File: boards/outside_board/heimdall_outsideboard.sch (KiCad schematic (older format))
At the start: 11 parts, among them J1 Conn_01x09, J2 Conn_01x06, Q1 2N3904, Q2 2N7000

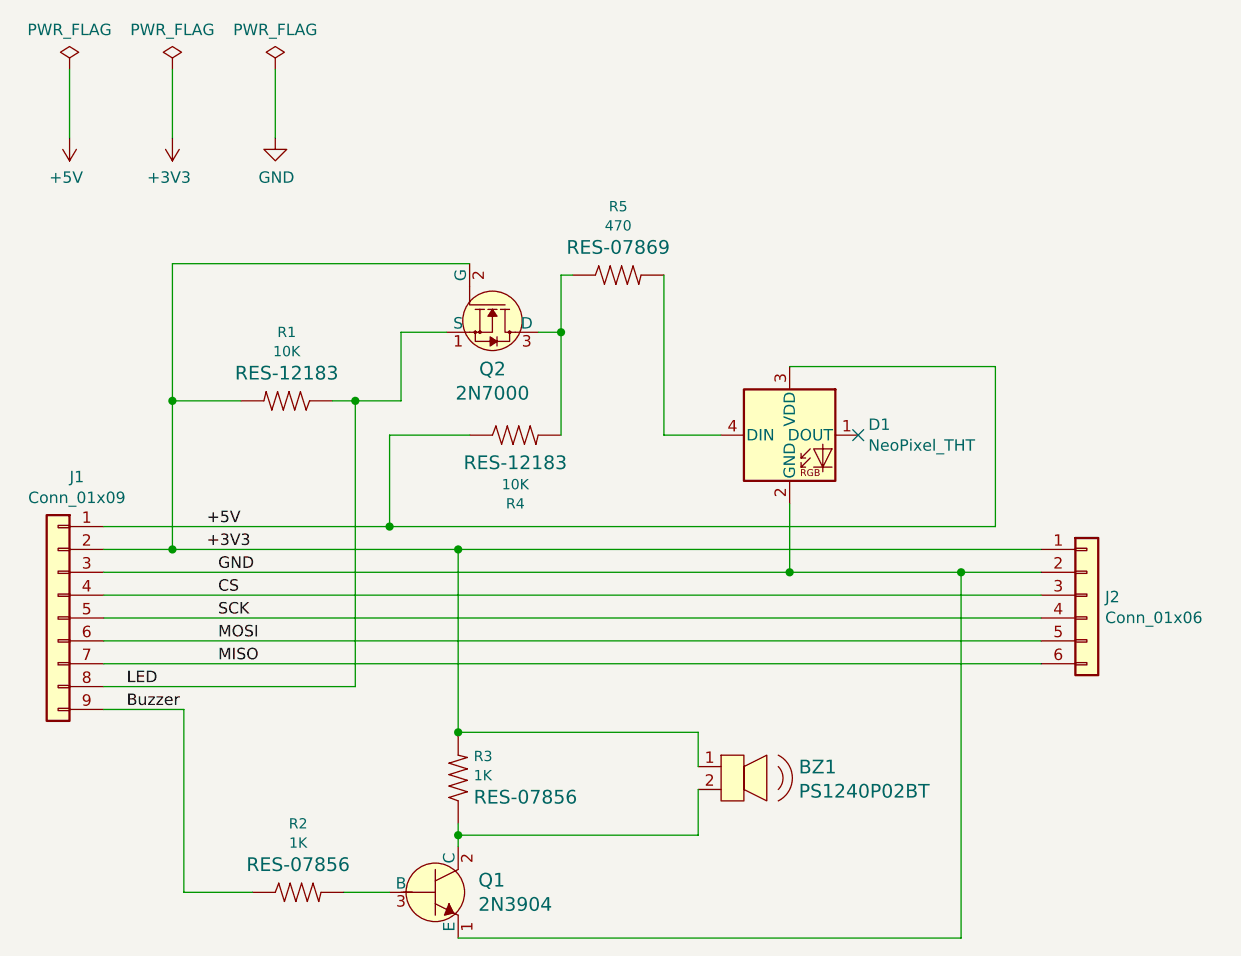
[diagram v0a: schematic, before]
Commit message: Update outside board schematics and layout to revision 2
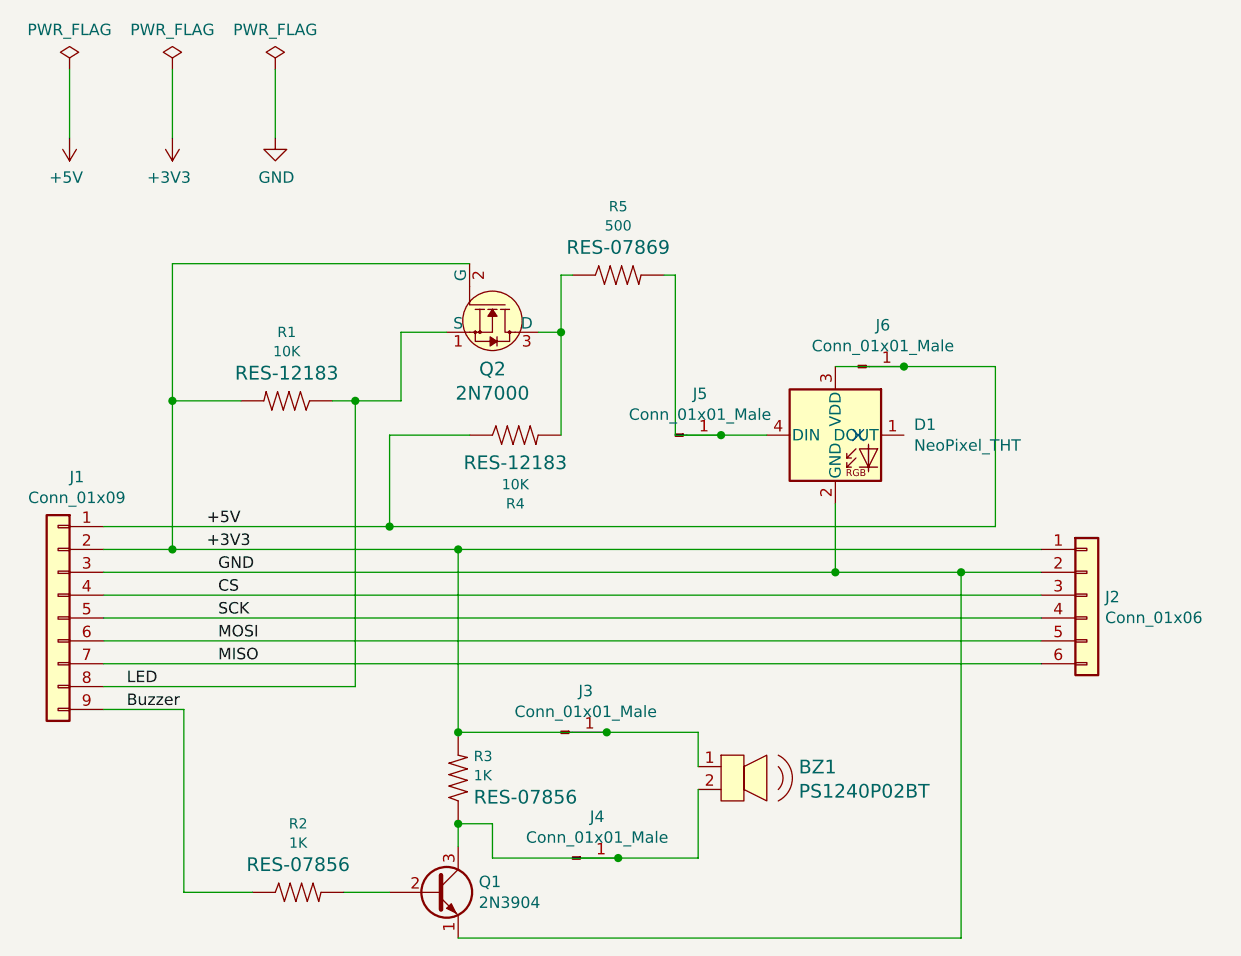
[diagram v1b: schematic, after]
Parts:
- removed Q1: 2N3904, Package_TO_SOT_THT:TO-92_Inline, symbol dk_Transistors-Bipolar-BJT-Single:2N3904
- added J3, J4, J5, J6: Conn_01x01_Male, Connector_PinHeader_2.54mm:PinHeader_1x01_P2.54mm_Vertical, symbol Connector:Conn_01x01_Male
- added Q1: 2N3904, Package_TO_SOT_THT:TO-92_Inline, symbol Transistor_BJT:2N3904
- D1: footprint LED:WS2812B -> LED_THT:LED_D5.0mm-4_RGB
- R5: value 470 -> 500
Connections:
- net +3V3: now also J3.1 (Pin_1)
- net +5V: now also J6.1 (Pin_1)
- net GND: now also Q1.1 (E)
- net at D1.4 (DIN), R5.2: now also J5.1 (Pin_1)
- net at BZ1.2, R3.1: now also J4.1 (Pin_1), Q1.3 (C)
- net at R2.2: now also Q1.2 (B)
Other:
- moved on the sheet: D1
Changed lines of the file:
@@
 Sheet 1 1
 Title "Heimdall Outside Board"
-Date "2020-07-24"
-Rev "01"
+Date "2020-11-07"
+Rev "02"
 Comp ""
 Comment1 "https://opensource.org/licenses/MIT"
@@
 L LED:NeoPixel_THT D1
 U 1 1 5F17E8A3
-P 4350 4950
-F 0 "D1" H 4694 4996 50  0000 L CNN
-F 1 "NeoPixel_THT" H 4694 4905 50  0000 L CNN
-F 2 "LED:WS2812B" H 4400 4650 50  0001 L TNN
-F 3 "https://www.adafruit.com/product/1938" H 4450 4575 50  0001 L TNN
-	1    4350 4950
+P 4550 4950
+F 0 "D1" H 4894 4996 50  0000 L CNN
+F 1 "NeoPixel_THT" H 4894 4905 50  0000 L CNN
+F 2 "LED_THT:LED_D5.0mm-4_RGB" H 4600 4650 50  0001 L TNN
+F 3 "https://www.adafruit.com/product/1938" H 4650 4575 50  0001 L TNN
+	1    4550 4950
 	1    0    0    -1
 $EndComp
@@
 	1700 6950 2000 6950
 Wire Wire Line
-	2900 6750 2900 6700
-Wire Wire Line
 	2900 6250 2900 5450
-Wire Wire Line
-	2900 6250 3950 6250
-Wire Wire Line
-	3950 6250 3950 6400
-Connection ~ 2900 6250
-Wire Wire Line
-	3950 6500 3950 6700
-Wire Wire Line
-	3950 6700 2900 6700
-Connection ~ 2900 6700
-Wire Wire Line
-	2900 6700 2900 6650
 Wire Wire Line
 	5100 7150 5100 5550
@@
 Connection ~ 3350 4500
 Wire Wire Line
-	3800 4250 3800 4950
-Wire Wire Line
-	3800 4950 4050 4950
-Wire Wire Line
 	2850 4500 2650 4500
-$Comp
-L SparkFun-Resistors:470OHM-0603-1_10W-1% R5
-U 1 1 5F209E6B
-P 3600 4250
-F 0 "R5" H 3600 4550 45  0000 C CNN
-F 1 "470" H 3600 4466 45  0000 C CNN
-F 2 "Resistor_THT:R_Axial_DIN0207_L6.3mm_D2.5mm_P10.16mm_Horizontal" H 3600 4400 20  0001 C CNN
-F 3 "" H 3600 4250 60  0001 C CNN
-F 4 "RES-07869" H 3600 4371 60  0000 C CNN "Field4"
-	1    3600 4250
-	1    0    0    -1
-$EndComp
 Wire Wire Line
 	1350 5450 1650 5450
@@
 Wire Wire Line
 	5250 5350 5250 4650
-Wire Wire Line
-	5250 4650 4350 4650
-Wire Wire Line
-	1350 5550 4350 5550
-Wire Wire Line
-	4350 5550 4350 5250
-Connection ~ 4350 5550
-Wire Wire Line
-	4350 5550 5100 5550
 $Comp
 L power:PWR_FLAG #FLG01
@@
 F 3 "~" H 2100 3350 50  0001 C CNN
 	1    2100 3350
-	1    0    0    -1
-$EndComp
-$Comp
-L dk_Transistors-Bipolar-BJT-Single:2N3904 Q1
-U 1 1 5F2401CC
-P 2800 6950
-F 0 "Q1" H 2988 7003 60  0000 L CNN
-F 1 "2N3904" H 2988 6897 60  0000 L CNN
-F 2 "Package_TO_SOT_THT:TO-92_Inline" H 3000 7150 60  0001 L CNN
-F 3 "https://my.centralsemi.com/get_document.php?cmp=1&mergetype=pd&mergepath=pd&pdf_id=LSSGP072.PDF" H 3000 7250 60  0001 L CNN
-F 4 "2N3904CS-ND" H 3000 7350 60  0001 L CNN "Digi-Key_PN"
-F 5 "2N3904" H 3000 7450 60  0001 L CNN "MPN"
-F 6 "Discrete Semiconductor Products" H 3000 7550 60  0001 L CNN "Category"
-F 7 "Transistors - Bipolar (BJT) - Single" H 3000 7650 60  0001 L CNN "Family"
-F 8 "https://my.centralsemi.com/get_document.php?cmp=1&mergetype=pd&mergepath=pd&pdf_id=LSSGP072.PDF" H 3000 7750 60  0001 L CNN "DK_Datasheet_Link"
-F 9 "/product-detail/en/central-semiconductor-corp/2N3904/2N3904CS-ND/4806876" H 3000 7850 60  0001 L CNN "DK_Detail_Page"
-F 10 "TRANS NPN 40V TO-92" H 3000 7950 60  0001 L CNN "Description"
-F 11 "Central Semiconductor Corp" H 3000 8050 60  0001 L CNN "Manufacturer"
-F 12 "Active" H 3000 8150 60  0001 L CNN "Status"
-	1    2800 6950
 	1    0    0    -1
 $EndComp
@@
 Wire Wire Line
 	2100 3350 2100 3650
+$Comp
+L Connector:Conn_01x01_Male J3
+U 1 1 5FA614DC
+P 3350 6250
+F 0 "J3" H 3458 6431 50  0000 C CNN
+F 1 "Conn_01x01_Male" H 3458 6340 50  0000 C CNN
+F 2 "Connector_PinHeader_2.54mm:PinHeader_1x01_P2.54mm_Vertical" H 3350 6250 50  0001 C CNN
+F 3 "~" H 3350 6250 50  0001 C CNN
+	1    3350 6250
+	1    0    0    -1
+$EndComp
+$Comp
+L Connector:Conn_01x01_Male J4
+U 1 1 5FA62088
+P 3400 6800
+F 0 "J4" H 3508 6981 50  0000 C CNN
+F 1 "Conn_01x01_Male" H 3508 6890 50  0000 C CNN
+F 2 "Connector_PinHeader_2.54mm:PinHeader_1x01_P2.54mm_Vertical" H 3400 6800 50  0001 C CNN
+F 3 "~" H 3400 6800 50  0001 C CNN
+	1    3400 6800
+	1    0    0    -1
+$EndComp
+$Comp
+L Connector:Conn_01x01_Male J5
+U 1 1 5FA690EE
+P 3850 4950
+F 0 "J5" H 3958 5131 50  0000 C CNN
+F 1 "Conn_01x01_Male" H 3958 5040 50  0000 C CNN
+F 2 "Connector_PinHeader_2.54mm:PinHeader_1x01_P2.54mm_Vertical" H 3850 4950 50  0001 C CNN
+F 3 "~" H 3850 4950 50  0001 C CNN
+	1    3850 4950
+	1    0    0    -1
+$EndComp
+$Comp
+L Connector:Conn_01x01_Male J6
+U 1 1 5FA69F83
+P 4650 4650
+F 0 "J6" H 4758 4831 50  0000 C CNN
+F 1 "Conn_01x01_Male" H 4758 4740 50  0000 C CNN
+F 2 "Connector_PinHeader_2.54mm:PinHeader_1x01_P2.54mm_Vertical" H 4650 4650 50  0001 C CNN
+F 3 "~" H 4650 4650 50  0001 C CNN
+	1    4650 4650
+	1    0    0    -1
+$EndComp
+Wire Wire Line
+	1350 5550 4550 5550
+Wire Wire Line
+	4550 5250 4550 5550
+Connection ~ 4550 5550
+Wire Wire Line
+	4550 5550 5100 5550
+Wire Wire Line
+	3850 4250 3800 4250
+Wire Wire Line
+	4050 4950 4250 4950
+Wire Wire Line
+	4850 4650 5250 4650
+Wire Wire Line
+	2900 6650 2900 6750
+Wire Wire Line
+	3950 6400 3950 6250
+Wire Wire Line
+	3950 6250 3550 6250
+Wire Wire Line
+	3550 6250 2900 6250
+Connection ~ 3550 6250
+Connection ~ 2900 6250
+Wire Wire Line
+	3950 6500 3950 6800
+Wire Wire Line
+	3950 6800 3600 6800
+Wire Wire Line
+	3600 6800 3050 6800
+Wire Wire Line
+	3050 6800 3050 6650
+Wire Wire Line
+	3050 6650 2900 6650
+Connection ~ 3600 6800
+Connection ~ 2900 6650
+Wire Wire Line
+	4850 4650 4550 4650
+Connection ~ 4850 4650
+Wire Wire Line
+	4050 4950 3850 4950
+Wire Wire Line
+	3850 4950 3850 4250
+Connection ~ 4050 4950
+$Comp
+L Transistor_BJT:2N3904 Q1
+U 1 1 5FA8FEA8
+P 2800 6950
+F 0 "Q1" H 2990 6996 50  0000 L CNN
+F 1 "2N3904" H 2990 6905 50  0000 L CNN
+F 2 "Package_TO_SOT_THT:TO-92_Inline" H 3000 6875 50  0001 L CIN
+F 3 "https://www.onsemi.com/pub/Collateral/2N3903-D.PDF" H 2800 6950 50  0001 L CNN
+	1    2800 6950
+	1    0    0    -1
+$EndComp
+$Comp
+L SparkFun-Resistors:470OHM-0603-1_10W-1% R5
+U 1 1 5F209E6B
+P 3600 4250
+F 0 "R5" H 3600 4550 45  0000 C CNN
+F 1 "500" H 3600 4466 45  0000 C CNN
+F 2 "Resistor_THT:R_Axial_DIN0207_L6.3mm_D2.5mm_P10.16mm_Horizontal" H 3600 4400 20  0001 C CNN
+F 3 "" H 3600 4250 60  0001 C CNN
+F 4 "RES-07869" H 3600 4371 60  0000 C CNN "Field4"
+	1    3600 4250
+	1    0    0    -1
+$EndComp
 $EndSCHEMATC
